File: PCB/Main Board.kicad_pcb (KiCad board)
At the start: 2 copper layers, 82.5 x 152.4 mm, 27 parts, among them IC1 MC34119, J1 Control_01, J2 Control_02, J3 UART, J4 Texas_DAC_Out, U1 EK-TM4C123GXL

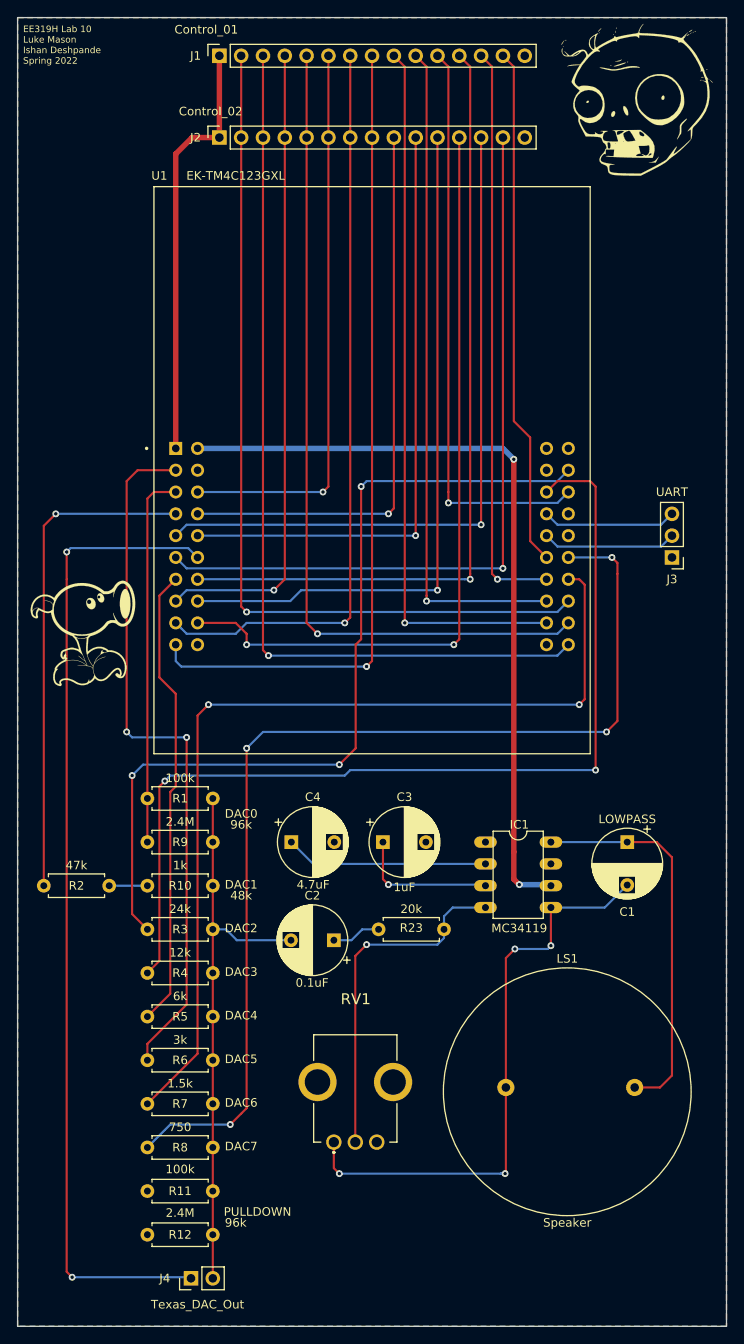
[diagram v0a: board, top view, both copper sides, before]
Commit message: generated gerbers and ordered PCB (#9)
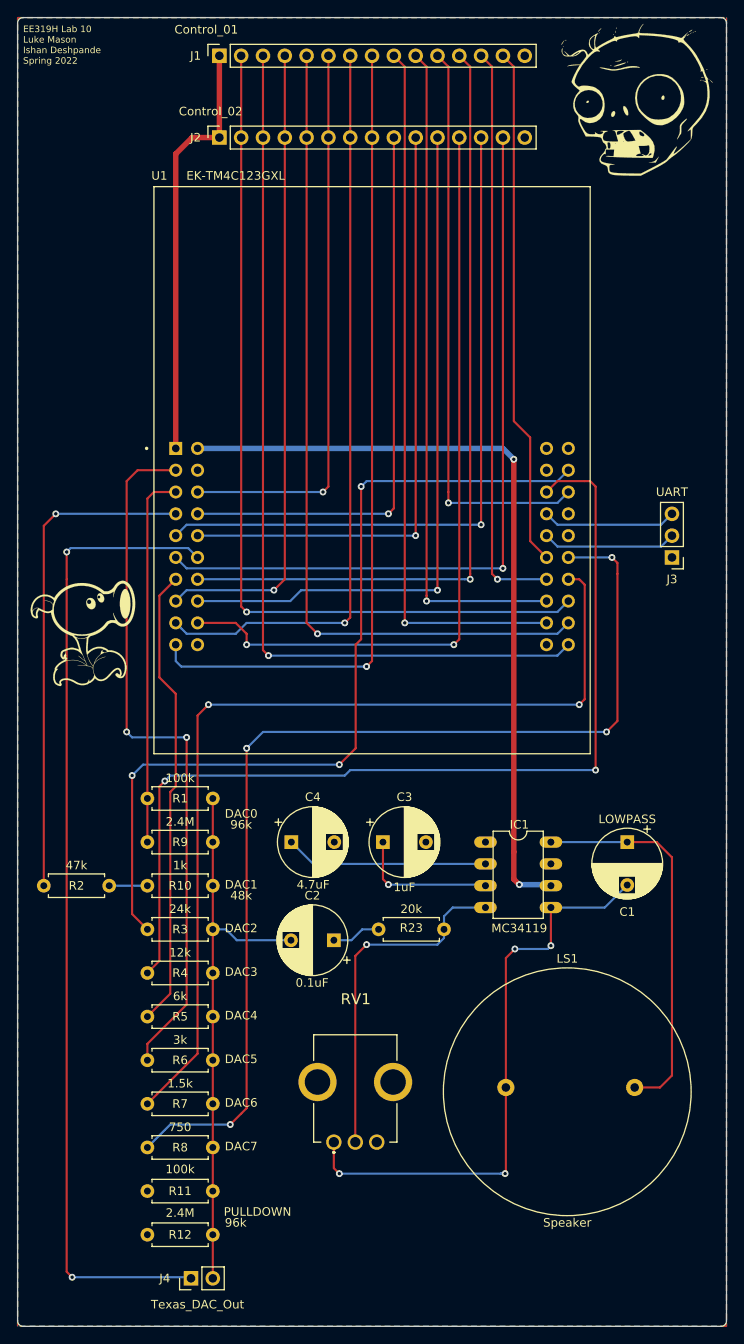
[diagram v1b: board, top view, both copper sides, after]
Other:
- outline, holes or cut-outs redrawn
